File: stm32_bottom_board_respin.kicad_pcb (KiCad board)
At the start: 2 copper layers, 90 x 60 mm, 51 parts, among them J1 Conn_01x02, J2 WS2812, J3 FAN_PWM, J4 SSR, J5 PURFUME, J6 Conn_01x14, J7 Conn_01x12, J8 Conn_01x12, Q1 2N3904(1AM), Q2 SS9013_J3, Q3 SS9013_J3, SW1 SW_Push, U1 74AHCT1G125, U2 OMRON-G3MB-202P, U3 STM32F103C8T6, U4 AMS1117-3.3, Y1 O8M, Y2 O32.768K

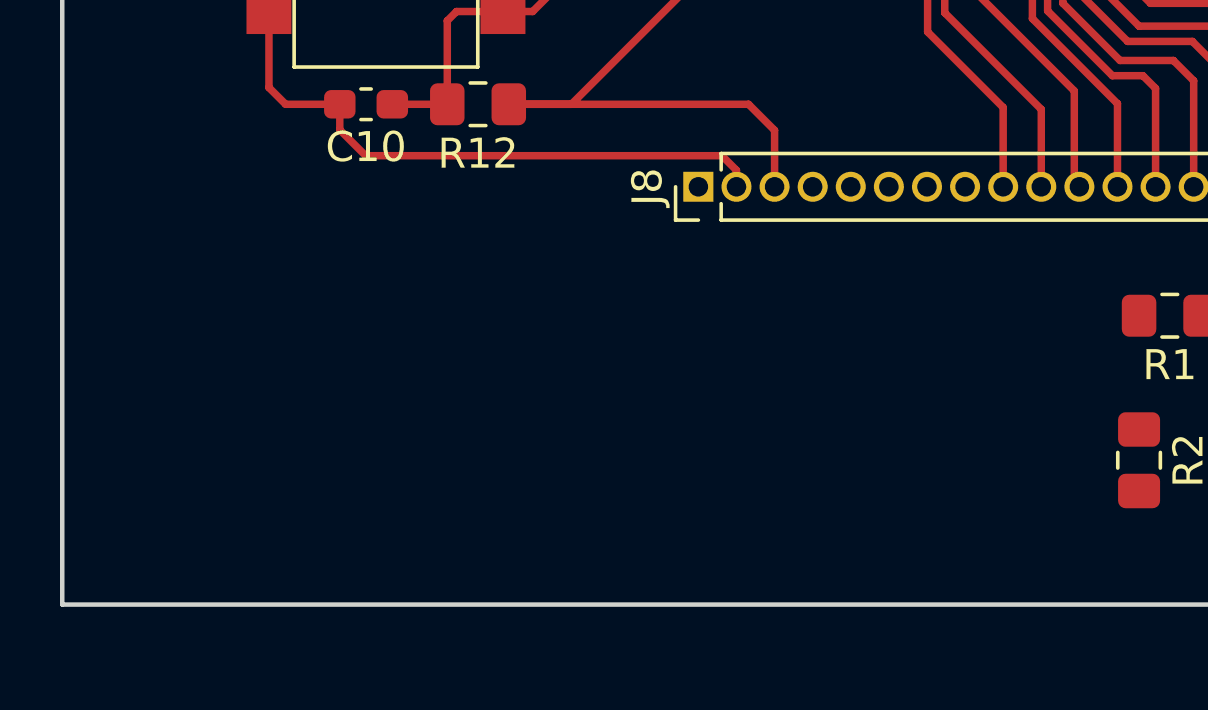
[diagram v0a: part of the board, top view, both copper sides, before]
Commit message: update,
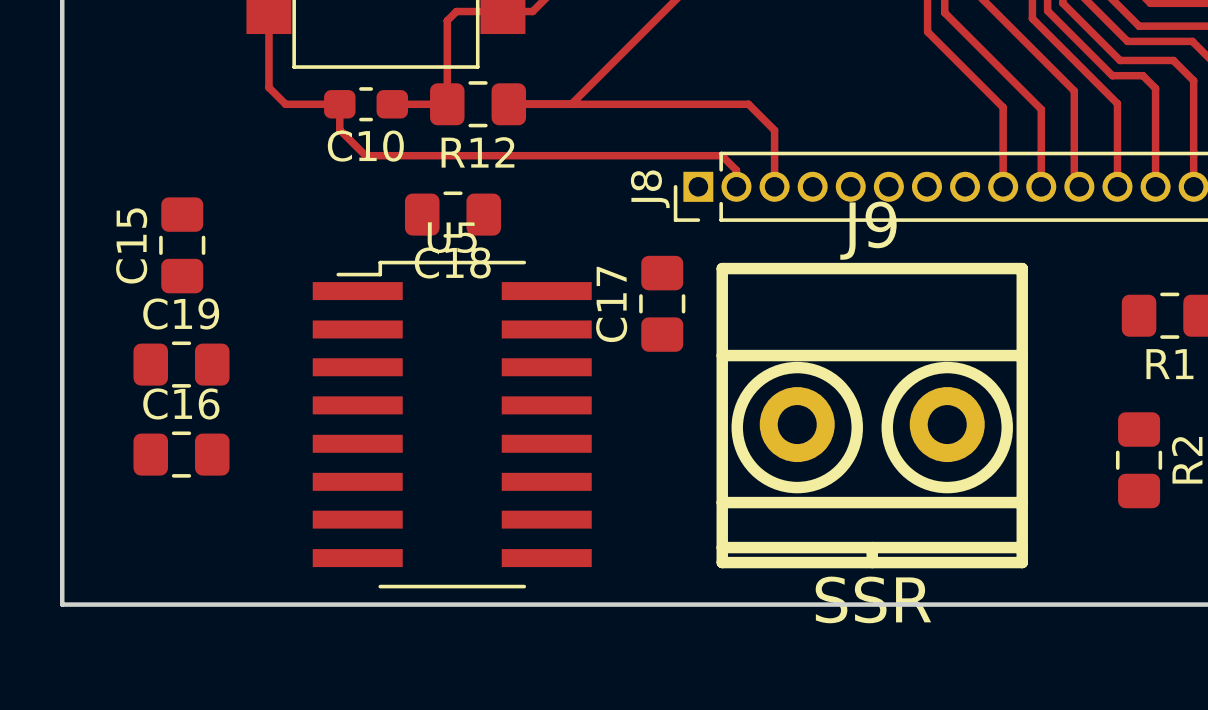
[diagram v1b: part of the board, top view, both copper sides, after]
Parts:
- added C15: C104, Capacitor_SMD:C_0805_2012Metric_Pad1.15x1.40mm_HandSolder, F.Cu at (9.00, 53.0)
- added C16: C104, Capacitor_SMD:C_0805_2012Metric_Pad1.15x1.40mm_HandSolder, F.Cu at (8.97, 60.0)
- added C17: C104, Capacitor_SMD:C_0805_2012Metric_Pad1.15x1.40mm_HandSolder, F.Cu at (25.0, 55.0)
- added C18: C104, Capacitor_SMD:C_0805_2012Metric_Pad1.15x1.40mm_HandSolder, F.Cu at (18.0, 52.0)
- added C19: C104, Capacitor_SMD:C_0805_2012Metric_Pad1.15x1.40mm_HandSolder, F.Cu at (8.97, 57.0)
- added J9: SSR, w_conn_mkds:mkds_1,5-2, F.Cu at (32.0, 59.0)
- added U5: SP3232EEN, footprint-lib:SOP-16_4.4x10.4mm_Pitch1.27mm, F.Cu at (18.0, 59.0)
